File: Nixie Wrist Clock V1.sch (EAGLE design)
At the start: 48 parts, among them Q1 310mA/60V/1.6Ω, Q2 310mA/60V/1.6Ω, Q3 310mA/60V/1.6Ω, Q4 310mA/60V/1.6Ω, Q5 310mA/60V/1.6Ω, U2 NRF52832, X3 32MHz, X4 32.768kHz

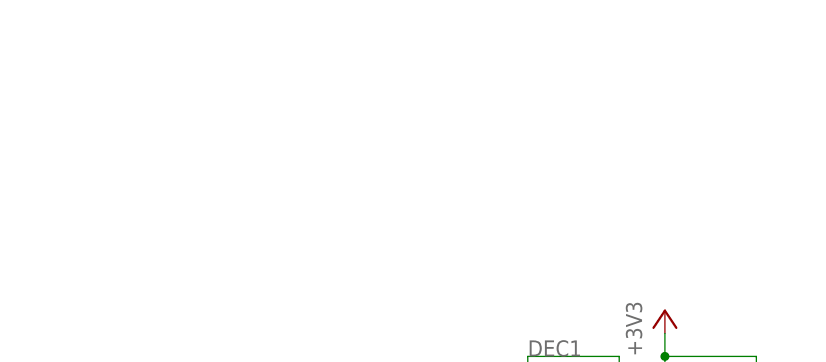
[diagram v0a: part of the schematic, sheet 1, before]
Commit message: Update #8
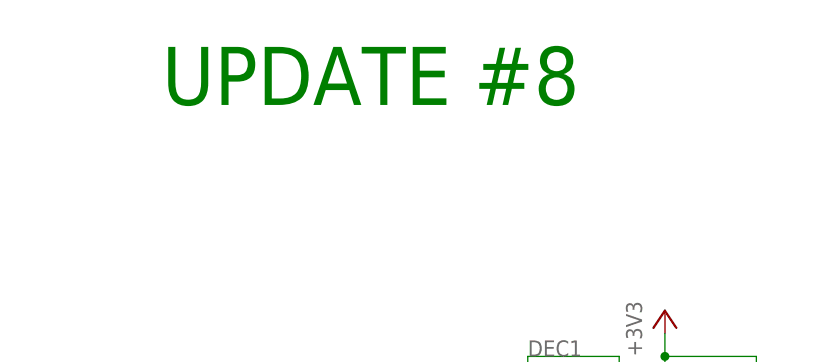
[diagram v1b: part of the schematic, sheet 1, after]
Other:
- note added: "UPDATE #8"
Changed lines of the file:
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@@
 <?xml version="1.0" encoding="utf-8"?>
 <!DOCTYPE eagle SYSTEM "eagle.dtd">
-<eagle version="9.5.0">
+<eagle version="9.5.1">
 <drawing>
 <settings>
@@
 <wire x1="20.32" y1="12.7" x2="43.18" y2="12.7" width="0.1524" layer="94"/>
 <text x="2.54" y="10.16" size="1.778" layer="94">In Progress</text>
+<text x="20.32" y="165.1" size="6.4516" layer="91">UPDATE #8</text>
 </plain>
 <instances>

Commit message: Revert "Update #8"
This reverts commit 503de56c1cec5e58df481c359deaf8b3a9d703f1.
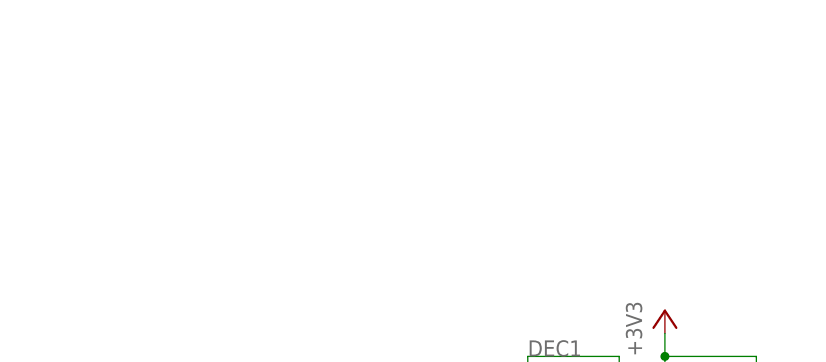
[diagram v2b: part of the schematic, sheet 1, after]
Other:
- note removed: "UPDATE #8"
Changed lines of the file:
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@@
 <?xml version="1.0" encoding="utf-8"?>
 <!DOCTYPE eagle SYSTEM "eagle.dtd">
-<eagle version="9.5.1">
+<eagle version="9.5.0">
 <drawing>
 <settings>
@@
 <wire x1="20.32" y1="12.7" x2="43.18" y2="12.7" width="0.1524" layer="94"/>
 <text x="2.54" y="10.16" size="1.778" layer="94">In Progress</text>
-<text x="20.32" y="165.1" size="6.4516" layer="91">UPDATE #8</text>
 </plain>
 <instances>
